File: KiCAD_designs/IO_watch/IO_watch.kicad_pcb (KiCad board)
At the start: 2 copper layers, 35 x 34.7 mm, 39 parts, among them U1 ATMEGA328P-AU, U2 DS3231S

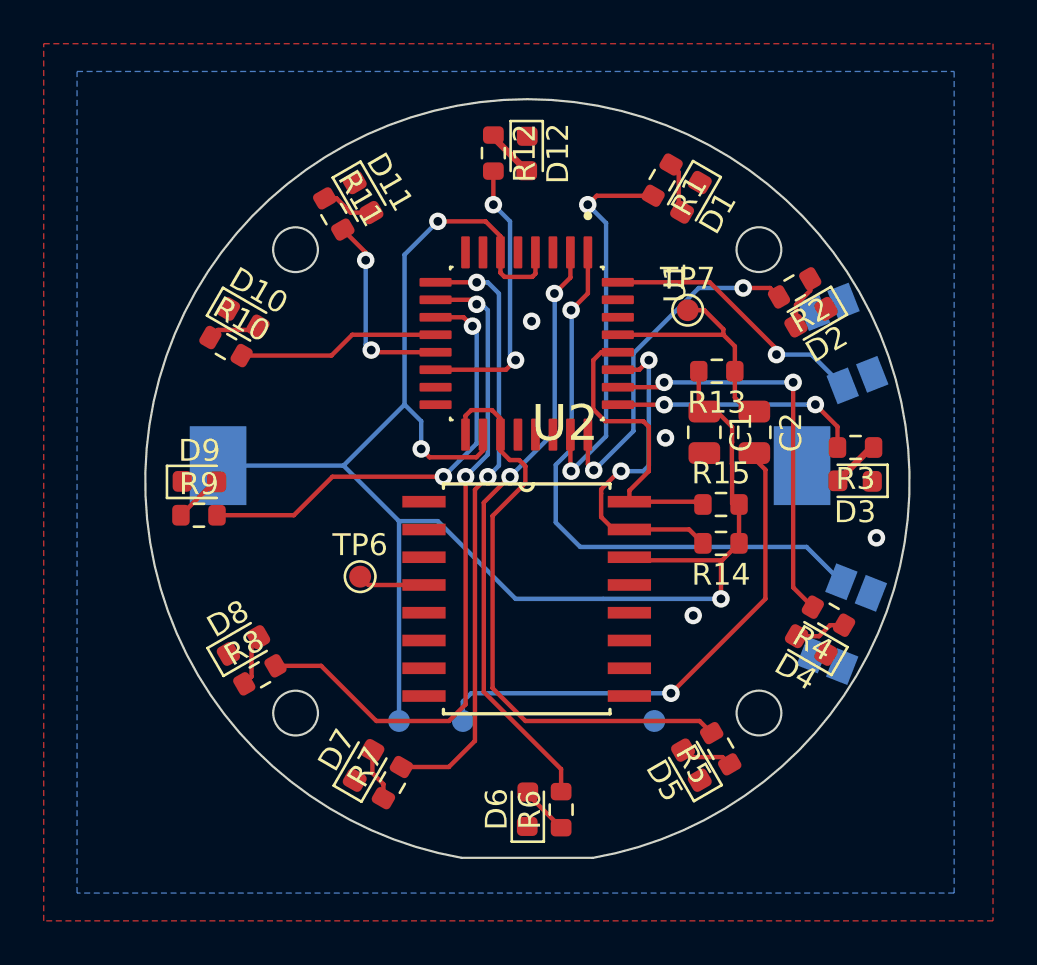
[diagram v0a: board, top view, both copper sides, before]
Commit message: ordered
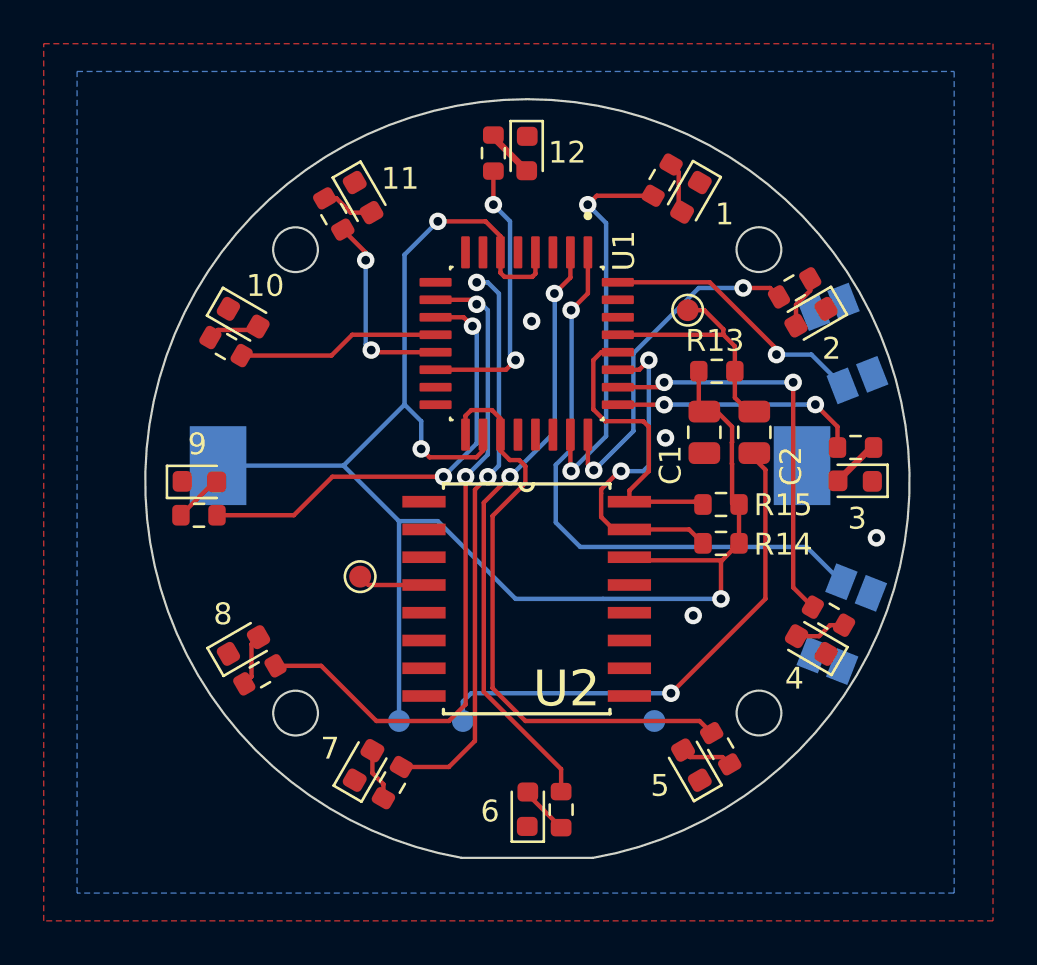
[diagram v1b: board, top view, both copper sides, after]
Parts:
- renumbered D1 to 1, D12 to 12, D2 to 2, D3 to 3, D4 to 4, D5 to 5
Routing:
- net /D5: track 27.9 -> 26.0 mm
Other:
- board text added: "1"
- board text added: "10"
- board text added: "11"
- board text added: "12"
- board text added: "2"
- board text added: "3"
- board text added: "4"
- board text added: "5"
- board text added: "6"
- board text added: "7"
- board text added: "8"
- board text added: "9"
